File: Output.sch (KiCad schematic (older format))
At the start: 12 parts, among them J4 Micro_SD_Card, J5 ST_01x02, Q1 DMN2230U

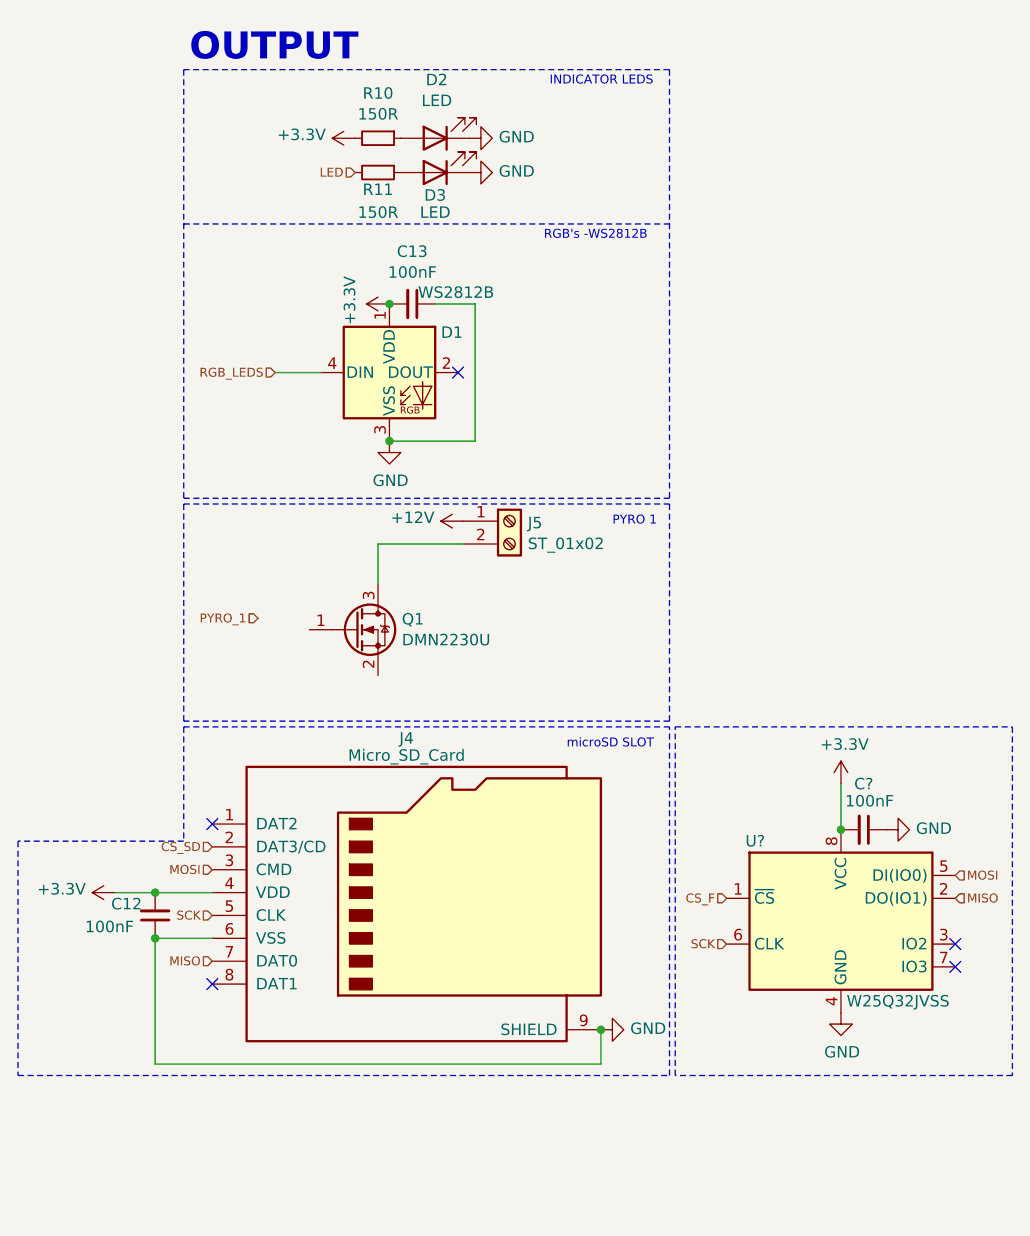
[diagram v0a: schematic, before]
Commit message: rc and cont on pyro, linear reg, flash
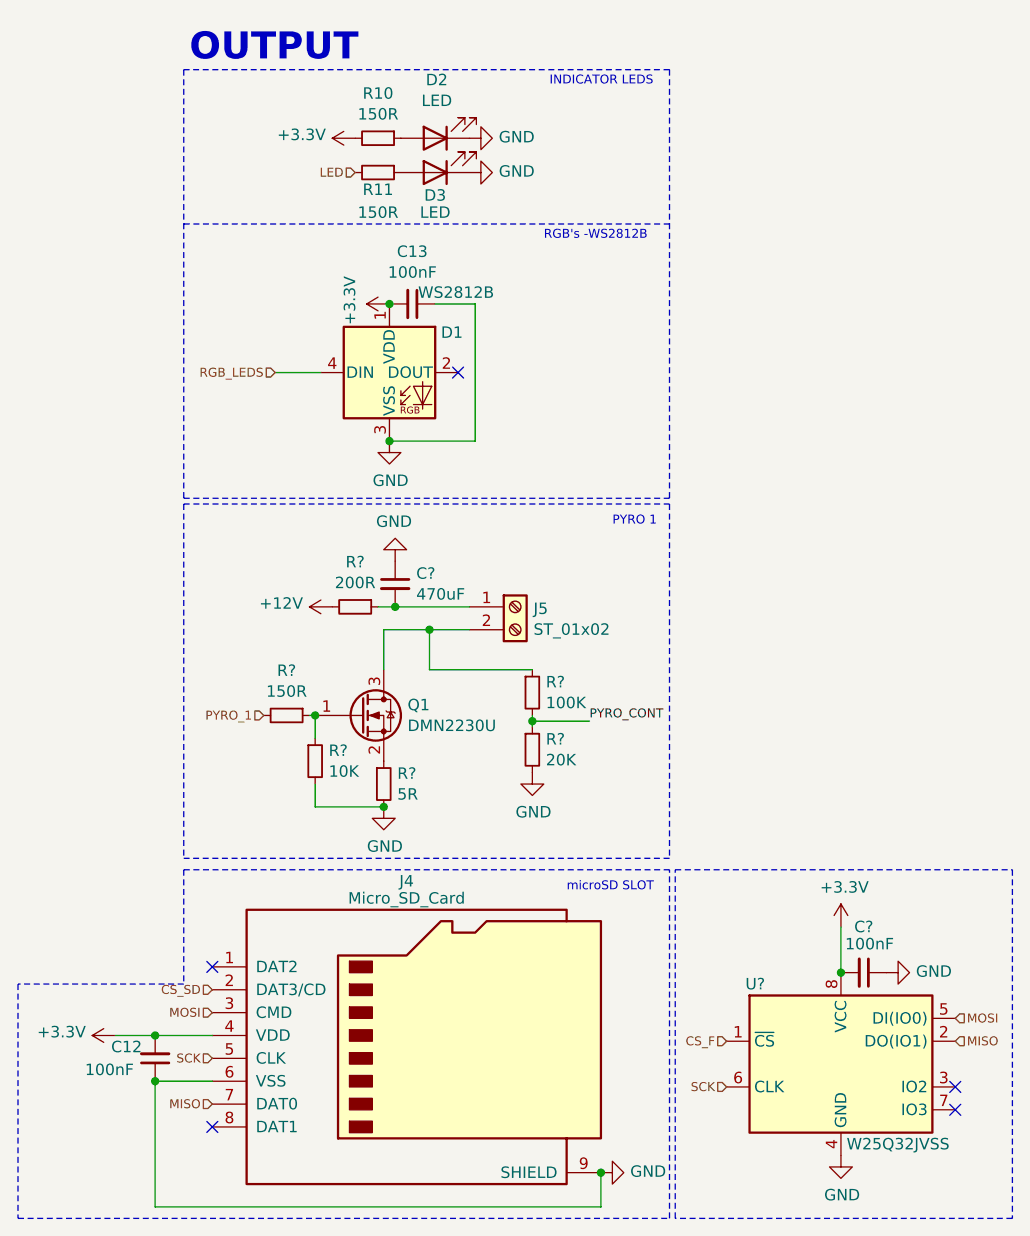
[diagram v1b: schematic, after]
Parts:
- added C?: 470uF, symbol Device:C_Small
- added R?: 100K, symbol Device:R_Small
- added R?: 20K, symbol Device:R_Small
- added R?: 10K, symbol Device:R_Small
- added R?: 200R, symbol Device:R_Small
- added R?: 150R, symbol Device:R_Small
- added R?: 5R, symbol Device:R_Small
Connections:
- net +12V: now also R?.2; no longer J5.1 (Pin_1)
- net GND: now also C?.1, R?.2, R?.2, R?.2
- net PYRO_1: now also R?.2
- net at Q1.1 (G): now also R?.1, R?.1
- net at Q1.2 (S): now also R?.1
- net at J5.2 (Pin_2), Q1.3 (D): now also R?.1
- new net: C?.2, J5.1 (Pin_1), R?.1
- new net PYRO_CONT: R?.1, R?.2
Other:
- moved on the sheet: C12, C?, J4, J5, Q1, U?
